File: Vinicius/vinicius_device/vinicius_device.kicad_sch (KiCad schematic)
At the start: 4 parts, among them J1 Connector, USB-TYPE-C-16P, U1 ESP32-C3, U2 CP2102-GMR, U3 VL53L0CXV0DH1

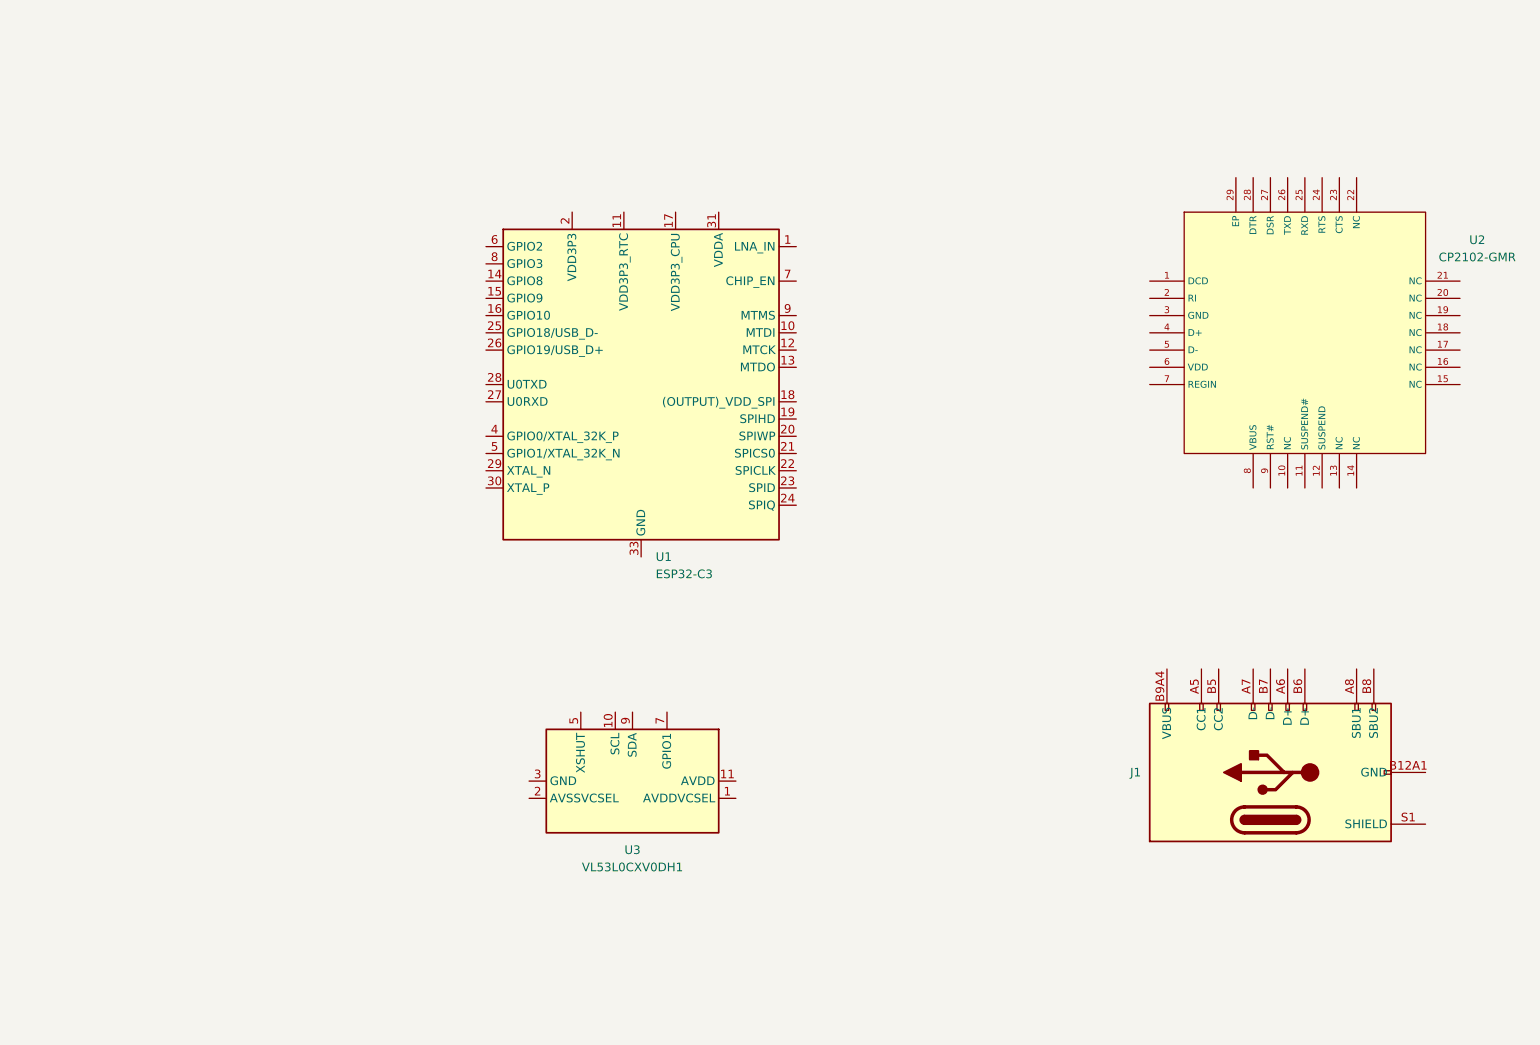
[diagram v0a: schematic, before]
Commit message: 6th, january. 2026
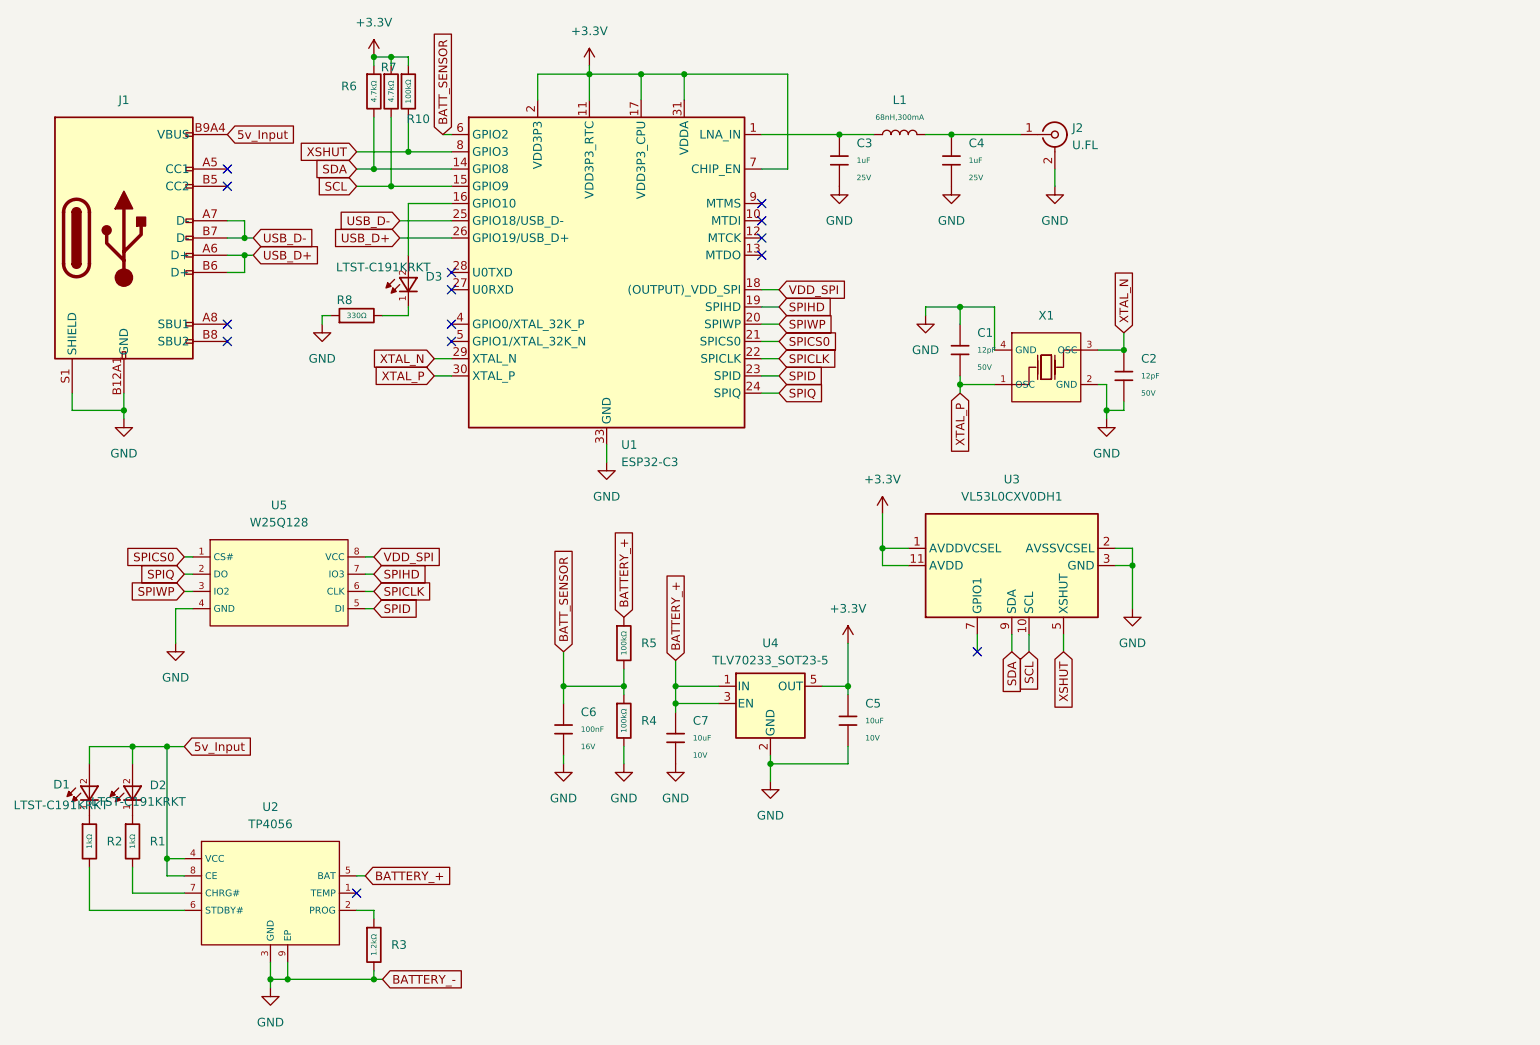
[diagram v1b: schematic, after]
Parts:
- removed U2: CP2102-GMR, PCM_JLCPCB:WQFN-28_L5.0-W5.0-P0.50-BL-EP3.2, symbol PCM_JLCPCB-Interface:Transceiver, USB
- added C1, C2: 12pF, PCM_JLCPCB:C_0402, symbol PCM_JLCPCB-Capacitors:0402,12pF
- added C3, C4: 1uF, PCM_JLCPCB:C_0402, symbol PCM_JLCPCB-Capacitors:0402,1uF
- added C5, C7: 10uF, PCM_JLCPCB:C_0603, symbol PCM_JLCPCB-Capacitors:0603,10uF
- added C6: 100nF, PCM_JLCPCB:C_0402, symbol PCM_JLCPCB-Capacitors:0402,100nF
- added D1, D2, D3: LTST-C191KRKT, LTST-C191KRKT:0603, symbol LTST-C191KRKT:LTST-C191KRKT
- added J2: U.FL, PCM_JLCPCB:IPEX-SMD_BWIPX-1-001E, symbol PCM_JLCPCB-Extended:RF, Connector, U.FL
- added L1: 68nH,300mA, PCM_JLCPCB:L_0603, symbol PCM_JLCPCB-Inductors:68nH,300mA
- added R1, R2: 1kΩ, PCM_JLCPCB:R_0402, symbol PCM_JLCPCB-Resistors:0402,1kΩ
- added R10, R4, R5: 100kΩ, PCM_JLCPCB:R_0402, symbol PCM_JLCPCB-Resistors:0402,100kΩ
- added R3: 1.2kΩ, PCM_JLCPCB:R_0402, symbol PCM_JLCPCB-Resistors:0402,1.2kΩ
- added R6, R7: 4.7kΩ, PCM_JLCPCB:R_0402, symbol PCM_JLCPCB-Resistors:0402,4.7kΩ
- added R8: 330Ω, PCM_JLCPCB:R_0402, symbol PCM_JLCPCB-Resistors:0402,330Ω
- added U2: TP4056, PCM_JLCPCB:ESOP-8_L4.9-W3.9-P1.27-LS6.0-BL-EP, symbol PCM_JLCPCB-Power:Battery, Li-Ion, 1.0A, TP4056
- added U4: TLV70233_SOT23-5, Package_TO_SOT_SMD:SOT-23-5, symbol Regulator_Linear:TLV70233_SOT23-5
- added U5: W25Q128, PCM_JLCPCB:SOIC-8_L5.3-W5.3-P1.27-LS8.0-BL, symbol PCM_JLCPCB-Memory:16MByte, SPI
- added X1: X322516MLB4SI, PCM_JLCPCB:OSC-SMD_4P-L3.2-W2.5-BL, symbol PCM_JLCPCB-Crystals:Crystal, 16MHz, 9pF
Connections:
- net GND: now reaches J1.A12B1 (GND), J1.B12A1 (GND)
- net GND: now also J1.S1 (SHIELD), U1.33 (GND), U3.12 (GND), U3.2 (AVSSVCSEL), U3.3 (GND), U3.4 (GND), U3.6 (GND), C1.2, C2.1, C3.2, C4.2, C5.2, C6.2, C7.2, J2.2 (Ext), R3.2, R4.2, R8.1, U2.3 (GND), U2.9 (EP), U4.2 (GND), U5.4 (GND), X1.2 (GND), X1.4 (GND)
- net USB_D+: now reaches J1.A6 (D+)
- net USB_D+: now also J1.B6 (D+), U1.26 (GPIO19/USB_D+)
- net USB_D-: now reaches J1.A7 (D-)
- net USB_D-: now also J1.B7 (D-), U1.25 (GPIO18/USB_D-)
- net 5v_Input: now reaches J1.A9B4 (VBUS), J1.B9A4 (VBUS)
- net 5v_Input: now also D1.2, D2.2, U2.4 (VCC), U2.8 (CE)
- net +3.3V: now reaches U3.1 (AVDDVCSEL)
- net +3.3V: now also U1.11 (VDD3P3_RTC), U1.17 (VDD3P3_CPU), U1.2 (VDD3P3), U1.3 (VDD3P3), U1.31 (VDDA), U1.32 (VDDA), U1.7 (CHIP_EN), U3.11 (AVDD), C5.1, R10.1, R6.1, R7.1, U4.5 (OUT)
- net SCL: now reaches U3.10 (SCL)
- net SCL: now also U1.15 (GPIO9), R7.2
- net XSHUT: now reaches U3.5 (XSHUT)
- net XSHUT: now also U1.8 (GPIO3), R10.2
- net SDA: now reaches U3.9 (SDA)
- net SDA: now also U1.14 (GPIO8), R6.2
- net at U1.1 (LNA_IN): now also C3.1, L1.1
- net at U1.16 (GPIO10): now also D3.2
- net VDD_SPI: now reaches U1.18 ((OUTPUT)_VDD_SPI)
- net VDD_SPI: now also U5.8 (VCC)
- net SPIHD: now reaches U1.19 (SPIHD)
- net SPIHD: now also U5.7 (IO3)
- net SPIWP: now reaches U1.20 (SPIWP)
- net SPIWP: now also U5.3 (IO2)
- net SPICS0: now reaches U1.21 (SPICS0)
- net SPICS0: now also U5.1 (CS#)
- net SPICLK: now reaches U1.22 (SPICLK)
- net SPICLK: now also U5.6 (CLK)
- net SPID: now reaches U1.23 (SPID)
- net SPID: now also U5.5 (DI)
- net SPIQ: now reaches U1.24 (SPIQ)
- net SPIQ: now also U5.2 (DO)
- net XTAL_N: now reaches U1.29 (XTAL_N)
- net XTAL_N: now also C2.2, X1.3 (OSC)
- net XTAL_P: now reaches U1.30 (XTAL_P)
- net XTAL_P: now also C1.1, X1.1 (OSC)
- net BATT_SENSOR: now reaches U1.6 (GPIO2)
- net BATT_SENSOR: now also C6.1, R4.1, R5.2
- new net: D3.1, R8.2
- new net: C4.1, J2.1 (In), L1.2
- new net: D2.1, R1.1
- new net: R3.1, U2.2 (PROG)
- new net: R2.2, U2.6 (STDBY#)
- new net: R1.2, U2.7 (CHRG#)
- new net: D1.1, R2.1
- new net BATTERY_+: C7.1, R5.1, U2.5 (BAT), U4.1 (IN), U4.3 (EN)
- no-connect marks 0 -> 14
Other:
- moved on the sheet: J1, U1, U3
